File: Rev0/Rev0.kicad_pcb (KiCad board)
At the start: 2 copper layers, 63 x 79.3 mm, 141 parts, among them J1 TERMBLOCK_1X2, J10 TERMBLOCK_1X2, J12 TERMBLOCK_1X2, J13 TERMBLOCK_1X2, J19 TERMBLOCK_1X2, J2 QWIIC_RIGHT_ANGLE, J20 TERMBLOCK_1X2, J21 TERMBLOCK_1X2, J22 TERMBLOCK_1X2, J23 TERMBLOCK_1X2, J24 TERMBLOCK_1X2, J25 TERMBLOCK_1X2, J26 TERMBLOCK_1X2, J28 Conn_01x02, J29 Conn_01x02, J3 QWIIC_RIGHT_ANGLE, J30 Conn_01x02, J31 Conn_01x02, J32 Conn_01x02, J33 Conn_01x02, J34 Conn_01x02, J35 Conn_01x02, J4 TERMBLOCK_1X2, J5 TERMBLOCK_1X2, J6 TERMBLOCK_1X2, J7 TERMBLOCK_1X2, J8 TERMBLOCK_1X2, J9 TERMBLOCK_1X2, Q1 AOD417, U1 PCA9685, U10 PC817, U11 PC817, U12 PC817, U13 PC817, U14 PC817, U15 PC817, U16 ADS1115IDGS, U17 ADS1115IDGS, U2 DRV8870DDA, U3 DRV8870DDA, U4 DRV8870DDA, U5 K7805-2000R3L, U6 TCA9406DC, U7 MCP23008-xSO, U8 PC817, U9 PC817

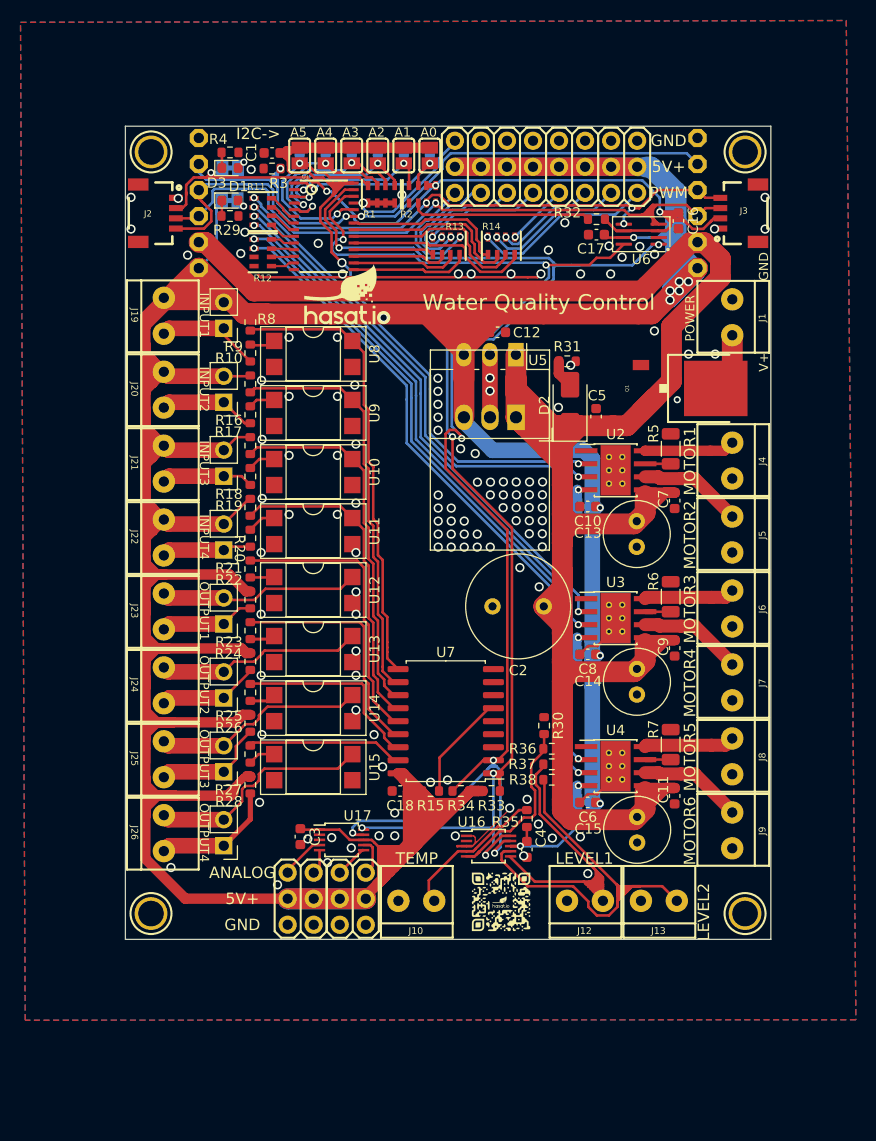
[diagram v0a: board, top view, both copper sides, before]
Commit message: .
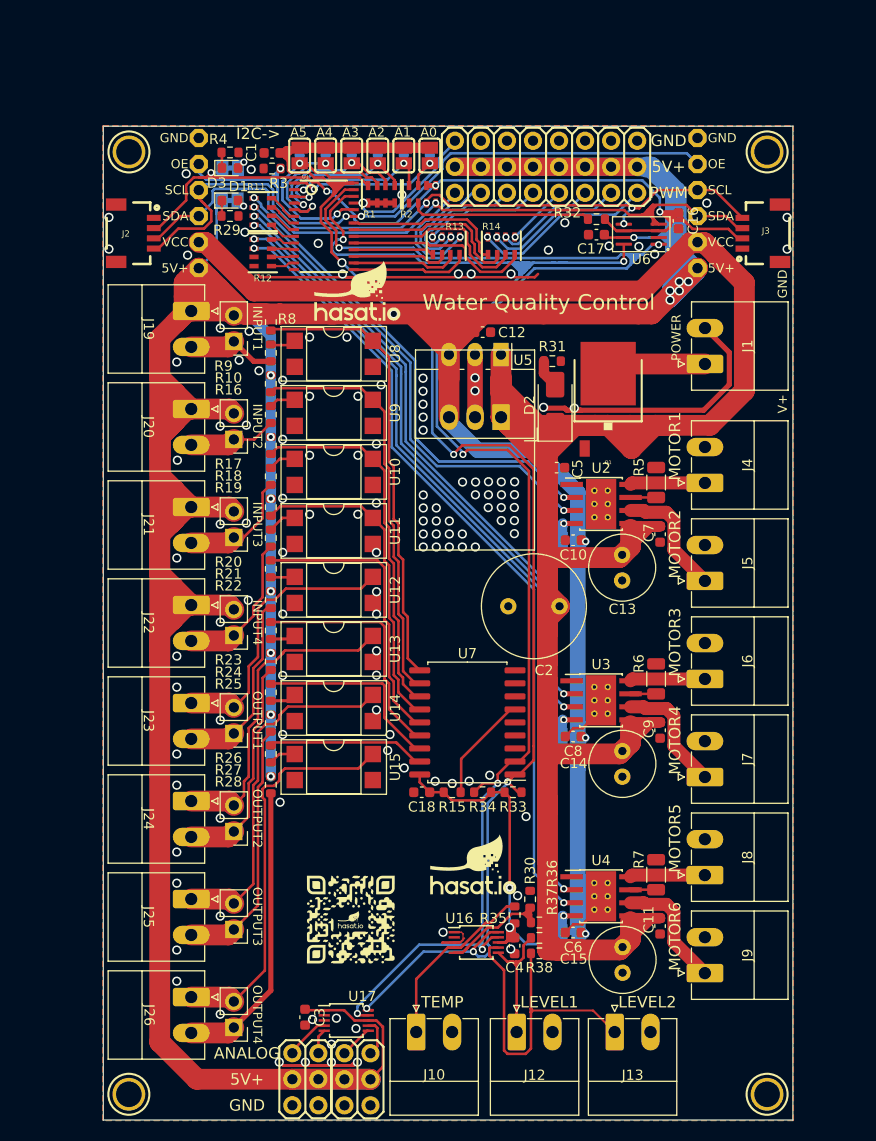
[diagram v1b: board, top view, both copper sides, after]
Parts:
- added G***: LOGO, Graphics:Hasatio_logo_micro, F.Cu at (145.8, 121.3)
- J1, J10, J12, J13, J19, J20, J21, J22, J23, J24, J25, J26, J4, J5, J6, J7, J8, J9: footprint Adafruit PCA9685 rev C:TERMBLOCK_1X2-3.5MM -> Connector_Phoenix_MC:PhoenixContact_MC_1,5_2-G-3.5_1x02_P3.50mm_Horizontal
- moved U$48 17.8 mm to (112.2, 143.7)
- moved J35 17.8 mm to (122.4, 137.2)
- moved U$e 17.8 mm to (174.4, 143.7)
- moved U17 17.6 mm to (133.4, 136.5)
- moved C3 17.6 mm to (129.4, 136.2)
- moved JP1 17.6 mm to (134.5, 142.2)
- moved JP2 17.6 mm to (129.4, 142.2)
- moved R30 17.0 mm to (151.3, 124.7)
- moved R36 17.0 mm to (152.2, 126.9)
- moved R37 17.0 mm to (152.2, 128.4)
- moved R38 17.0 mm to (152.2, 130.0)
- moved J26 16.3 mm to (118.3, 134.2)
- moved J34 15.4 mm to (122.4, 127.6)
- moved G*** 14.8 mm to (133.8, 126.7) (x2)
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- renumbered U$50 to U$e
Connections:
- J1 pad 1: GND -> Net-(Q1-D)
- J1 pad 2: Net-(Q1-D) -> GND
- J19 pad 1: /I1 -> +5V
- J19 pad 2: +5V -> /I1
- J20 pad 1: /I2 -> +5V
- J20 pad 2: +5V -> /I2
- J21 pad 1: /I3 -> +5V
- J21 pad 2: +5V -> /I3
- J22 pad 1: /I4 -> +5V
- J22 pad 2: +5V -> /I4
- J23 pad 1: /O1B -> /O1A
- J23 pad 2: /O1A -> /O1B
- J24 pad 1: /O2B -> /O2A
- J24 pad 2: /O2A -> /O2B
- J25 pad 1: /O3B -> /O3A
- J25 pad 2: /O3A -> /O3B
- J26 pad 1: /O4B -> /O4A
- J26 pad 2: /O4A -> /O4B
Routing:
- net +5V: track 743.2 -> 637.2 mm, vias 12 -> 20
- net VCC: track 239.3 -> 292.7 mm
- net GND: track 88.7 -> 132.6 mm, vias 125 -> 129
- net /Ain2: track 40.5 -> 13.4 mm
- net /SCL_B: track 127.2 -> 153.5 mm
- net /SDA_B: track 142.0 -> 159.3 mm
- net /O4A: track 22.3 -> 38.9 mm
- net /O4B: track 13.0 -> 28.9 mm
- net /O3A: track 20.8 -> 34.9 mm
- net /O3B: track 12.0 -> 25.2 mm
- net /Ain3: track 46.3 -> 33.3 mm
- net /P4: track 64.5 -> 76.6 mm
- net /P5: track 65.9 -> 78.0 mm
- net /O2B: track 10.5 -> 21.8 mm
- net /O2A: track 20.1 -> 31.1 mm
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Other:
- board size 63 x 79.3 mm -> 67.3 x 96.9 mm
